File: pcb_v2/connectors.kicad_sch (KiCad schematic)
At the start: 15 parts, among them J1 RJ45, J2 RJ45, J5 Screw_Terminal_01x03, U1 VL53L0CXV0DH1

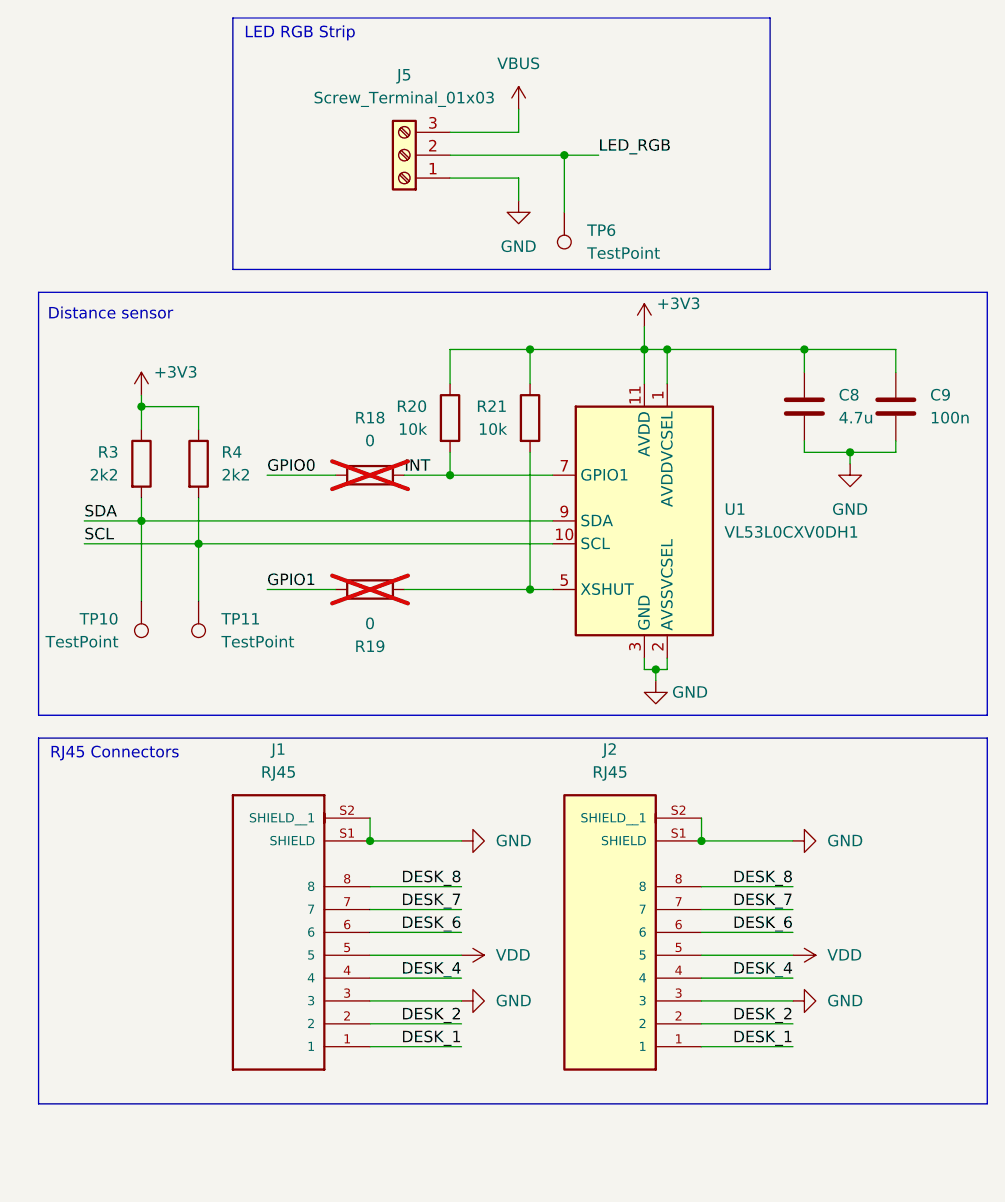
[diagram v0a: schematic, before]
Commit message: Replace schematic RJ45 with symbol from the library
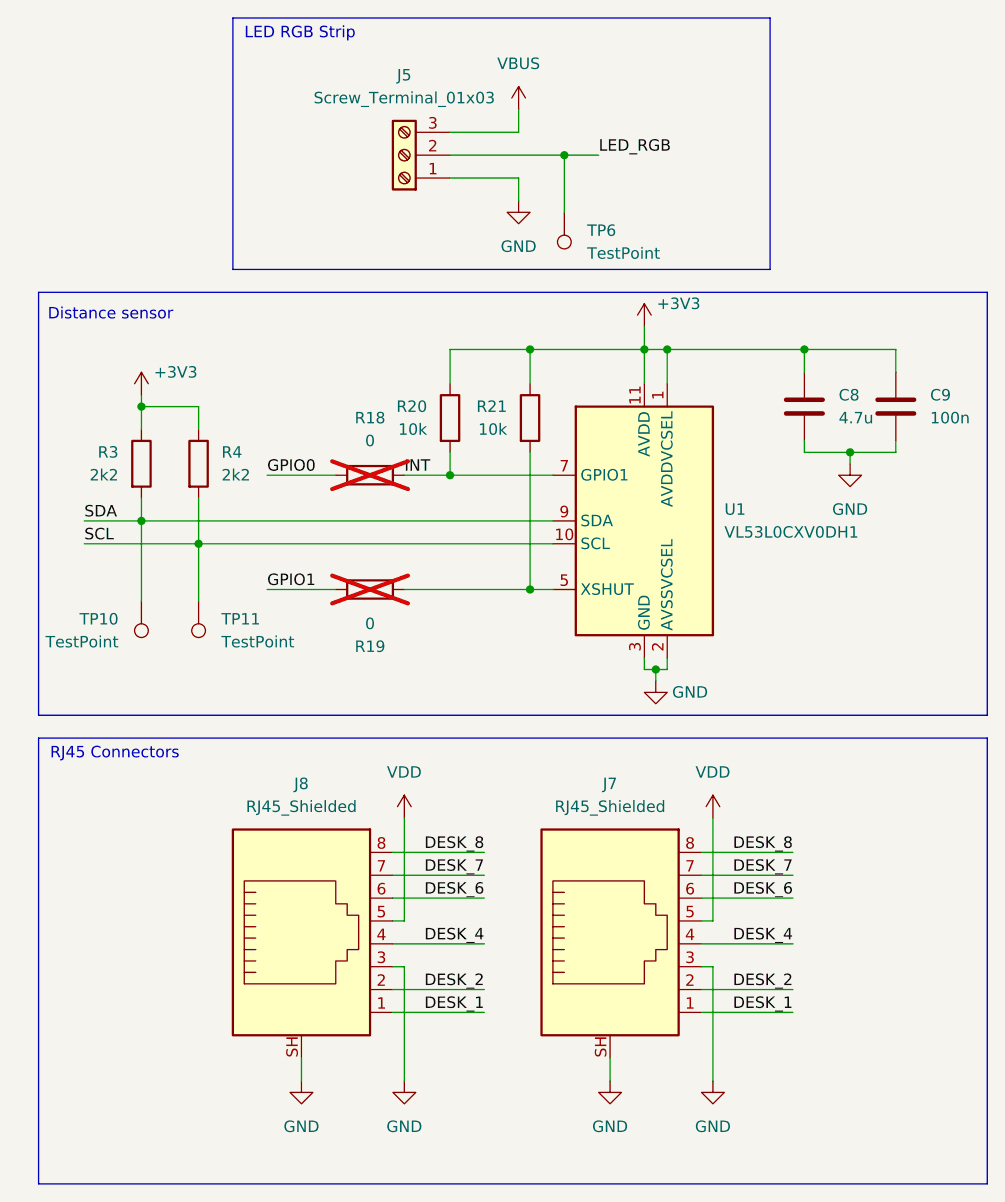
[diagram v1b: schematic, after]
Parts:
- removed J1, J2: RJ45, Connector_RJ:RJ45_Amphenol_54602-x08_Horizontal, symbol A-2004-2-4-LPS-N-R:A-2004-2-4-LPS-N-R
- added J7, J8: RJ45_Shielded, Connector_RJ:RJ45_Amphenol_54602-x08_Horizontal, symbol Connector:RJ45_Shielded
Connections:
- net DESK_1: now also J7.1, J8.1
- net DESK_2: now also J7.2, J8.2
- net DESK_4: now also J7.4, J8.4
- net DESK_6: now also J7.6, J8.6
- net DESK_7: now also J7.7, J8.7
- net DESK_8: now also J7.8, J8.8
- net GND: now also J7.3, J7.SH, J8.3, J8.SH
- net VDD: now also J7.5, J8.5
